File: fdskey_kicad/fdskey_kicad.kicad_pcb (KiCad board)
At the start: 2 copper layers, 70 x 18.1 mm, 15 parts, among them J2 Micro_SD_Card, J3 ISP_HEADER, J4 DISPLAY, SW1 SW_Push, SW2 SW_Push, SW3 SW_Push, SW4 SW_Push, U1 STM32G0B0CETx, U2 LD1117S33TR_SOT223

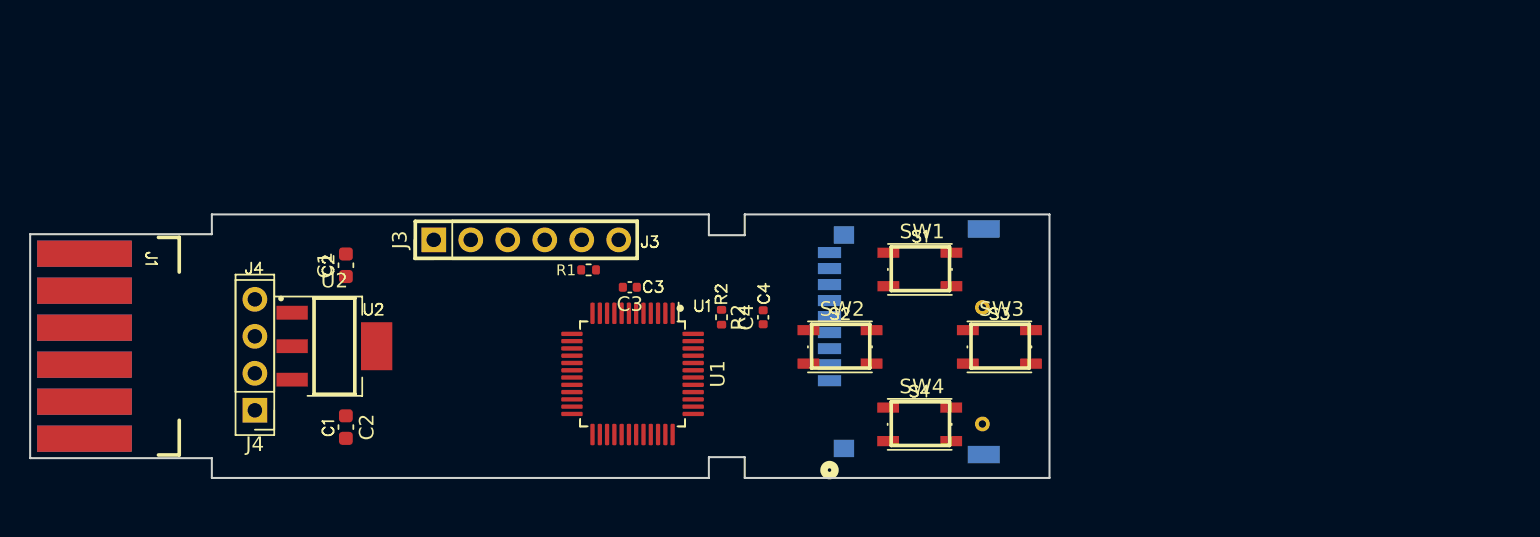
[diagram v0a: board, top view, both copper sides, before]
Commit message: (mostly) passes DRC!
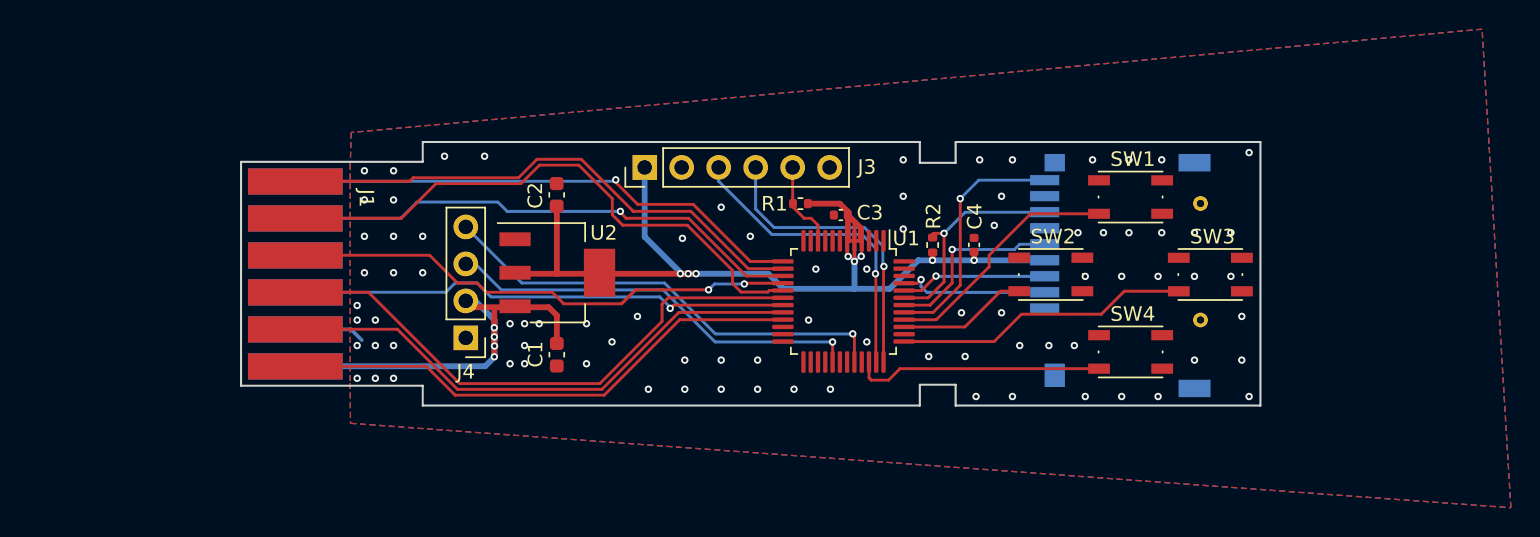
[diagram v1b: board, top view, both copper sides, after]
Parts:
- added J1: FDS_RAM_ADAPTER, Connector_PCBEdge:edgeconn_100mil_2x6, F.Cu at (118.3, 99.1)
- J2: footprint sdcard:112J-TDAR-R01_ATT -> sdcard:112J-TDAR-R01_ATT_fdskey
- U2: footprint Package_TO_SOT_SMD:SOT-223-3_TabPin2 -> Package_TO_SOT_SMD:SOT-223-3_TabPin2_fdskey
- moved C2 21.5 mm to (136.2, 93.7), turned to 90 degrees
- moved U2 16.1 mm to (136.2, 99.0)
- moved C1 15.7 mm to (136.2, 104.6), turned to -90 degrees
- moved R2 15.3 mm to (162.0, 97.1)
- moved C3 15.3 mm to (155.7, 95.0)
- moved U1 15.3 mm to (155.9, 101.0)
- moved SW4 15.3 mm to (175.6, 104.4)
- moved J3 15.3 mm to (142.2, 91.8)
- moved J4 15.3 mm to (130.0, 103.5)
- moved SW3 15.3 mm to (181.1, 99.1)
- moved C4 15.3 mm to (164.9, 97.1)
- moved SW2 15.3 mm to (170.1, 99.1)
- moved J2 15.3 mm to (169.4, 101.4)
- moved SW1 15.3 mm to (175.6, 93.8)
- moved R1 15.2 mm to (152.9, 94.3)
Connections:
- C1 pad 1: +3V3 -> +5V
- C2 pad 1: +5V -> +3V3
- U1 pad 13: unconnected-(U1-PA2-Pad13) -> /~{STOP_MOTOR}
- U1 pad 14: unconnected-(U1-PA3-Pad14) -> /~{READY}
- U1 pad 15: unconnected-(U1-PA4-Pad15) -> /~{MEDIA_SET}
- U1 pad 16: unconnected-(U1-PA5-Pad16) -> /~{WRITABLE_MEDIA}
- U1 pad 17: unconnected-(U1-PA6-Pad17) -> /READ_DATA
- U1 pad 18: unconnected-(U1-PA7-Pad18) -> /WRITE_DATA
- U1 pad 19: unconnected-(U1-PB0-Pad19) -> /MOTOR_ON
- U1 pad 20: unconnected-(U1-PB1-Pad20) -> /~{SCAN_MEDIA}
- U1 pad 21: unconnected-(U1-PB2-Pad21) -> /~{WRITE}
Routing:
- net +3V3: track 0.00 -> 70.3 mm, vias 0 -> 8
- net /READ_DATA: track 0.00 -> 39.8 mm
- net /WRITE_DATA: track 0.00 -> 39.2 mm
- net /~{SCAN_MEDIA}: track 0.00 -> 37.4 mm
- net /~{READY}: track 0.00 -> 37.3 mm
- net /~{WRITABLE_MEDIA}: track 0.00 -> 36.7 mm, vias 0 -> 2
- net /~{WRITE}: track 0.00 -> 36.5 mm
- net /~{MEDIA_SET}: track 0.00 -> 36.1 mm, vias 0 -> 1
- net /~{STOP_MOTOR}: track 0.00 -> 35.9 mm, vias 0 -> 1
- net /MOTOR_ON: track 0.00 -> 34.6 mm, vias 0 -> 1
- net I2C_SDA: track 0.00 -> 31.6 mm, vias 0 -> 1
- net +5V: track 0.00 -> 30.5 mm, vias 0 -> 4
- net I2C_SCL: track 0.00 -> 28.1 mm, vias 0 -> 1
- net SWDIO: track 0.00 -> 21.4 mm, vias 0 -> 1
- net SWCLK: track 0.00 -> 20.7 mm, vias 0 -> 1
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- added copper zone on B.Cu, net GND
- added copper zone on F.Cu, net GND
